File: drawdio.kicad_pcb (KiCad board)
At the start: 2 copper layers, 45.7 x 12.7 mm, 12 parts, among them P1 CONN_2, P2 CONN_01X01, Q1 BC558, Q2 BC547, U1 LM555N

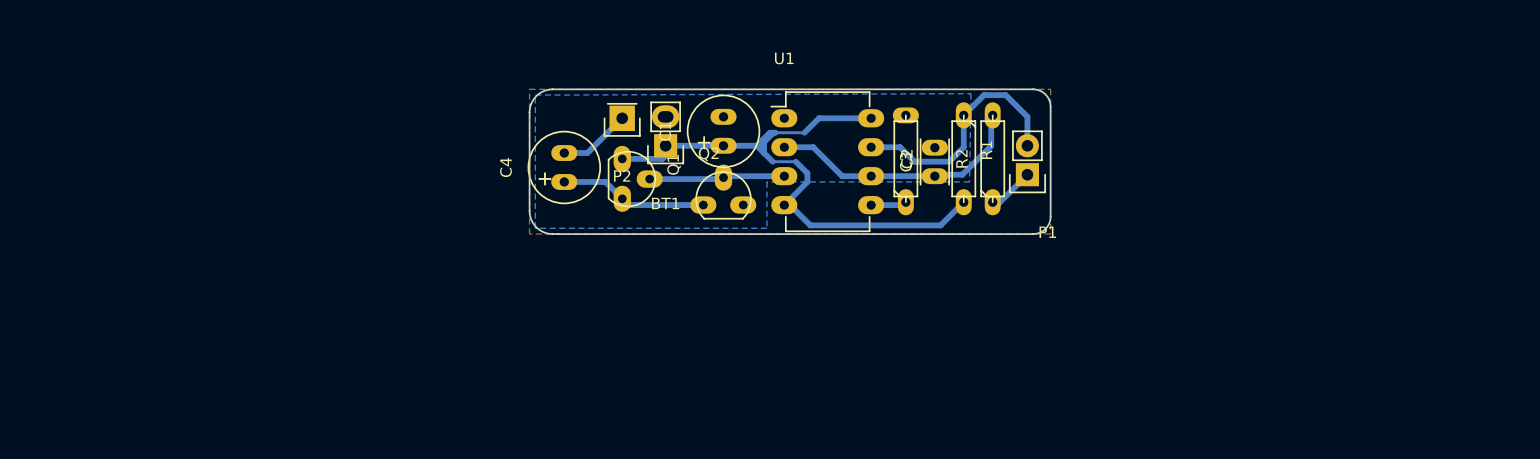
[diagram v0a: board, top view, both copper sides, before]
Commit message: Heavy work
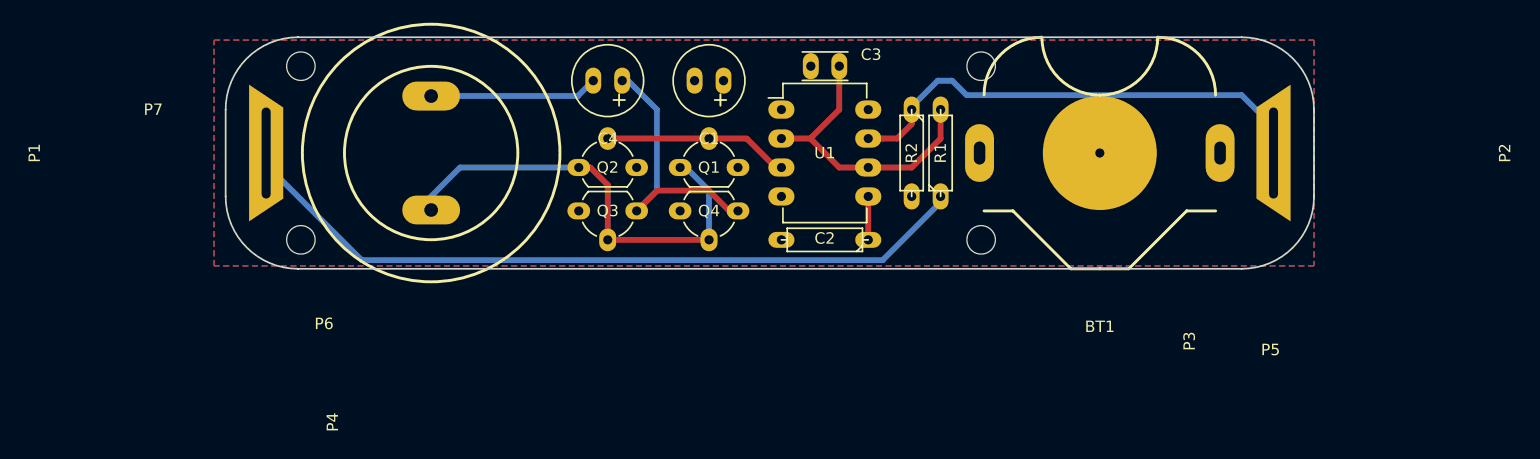
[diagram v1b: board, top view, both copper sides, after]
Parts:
- added P3: CONN_01X01, Mounting_Holes:MountingHole_2-5mm, F.Cu at (120.4, 94.0)
- added P4: CONN_01X02, drawdio:RS_mini_speaker_724-3100, F.Cu at (72.1, 86.4)
- added P5: CONN_01X01, Mounting_Holes:MountingHole_2-5mm, F.Cu at (120.4, 78.7)
- added P6: CONN_01X01, Mounting_Holes:MountingHole_2-5mm, F.Cu at (60.7, 94.0)
- added P7: CONN_01X01, Mounting_Holes:MountingHole_2-5mm, F.Cu at (60.7, 78.7)
- added Q3: BC558, Housings_TO-92:TO-92_Molded_Wide_Oval, F.Cu at (90.2, 91.4)
- added Q4: BC547, Housings_TO-92:TO-92_Molded_Wide_Oval, F.Cu at (99.1, 91.4)
- BT1: footprint Pin_Headers:Pin_Header_Straight_1x02 -> drawdio:CR2025_Keystone_3002_button_cell_holder_SMT
- P1: value CONN_2 -> CONN_01X01; footprint Pin_Headers:Pin_Header_Straight_1x02 -> drawdio:Drawdio_conn
- P2: footprint Pin_Headers:Pin_Header_Straight_1x01 -> drawdio:Drawdio_conn
- Q1, Q2: footprint drawdio:TO-92_JorFru_compact -> Housings_TO-92:TO-92_Molded_Wide_Oval
- moved P1 66.8 mm to (57.7, 86.4), turned to 270 degrees
- moved P2 57.2 mm to (146.1, 86.4), turned to 90 degrees
- moved BT1 38.1 mm to (130.8, 86.4), turned to 0 degrees
- moved C3 12.8 mm to (108.0, 78.7), turned to 180 degrees
- moved Q2 11.8 mm to (85.1, 87.6)
- moved C4 10.2 mm to (88.9, 80.0), turned to 180 degrees
- moved C2 10.1 mm to (106.7, 94.0), turned to 180 degrees
- moved C1 5.71 mm to (97.8, 80.0), turned to 180 degrees
- moved R1 4.60 mm to (116.8, 86.4)
- moved R2 4.60 mm to (114.3, 86.4)
- moved Q1 4.58 mm to (94.0, 87.6), turned to 0 degrees
- moved U1 0.80 mm to (102.9, 82.5)
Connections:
- P2 pad 1: Net-(C4-Pad2) -> Net-(P2-Pad1)
- Q1 pad 1: VCC -> Net-(P4-Pad2)
- Q1 pad 3: Net-(C4-Pad1) -> VCC
- Q2 pad 1: Net-(C4-Pad1) -> Net-(P4-Pad2)
- R2 pad 1: Net-(P1-Pad2) -> Net-(P2-Pad1)
- U1 pad 7: Net-(P1-Pad2) -> Net-(P2-Pad1)
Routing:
- net Net-(P1-Pad1): track 4.23 -> 66.7 mm
- net VCC: track 54.7 -> 0.00 mm
- net Net-(P2-Pad1): track 0.00 -> 50.9 mm
- net Net-(P4-Pad2): track 0.00 -> 40.2 mm
- net Net-(P1-Pad2): track 21.9 -> 0.00 mm
- net Net-(C4-Pad1): track 13.0 -> 24.1 mm
- net Net-(C4-Pad2): track 6.34 -> 15.8 mm
- net Net-(Q1-Pad2): track 13.3 -> 16.8 mm
- net Net-(C3-Pad1): track 23.6 -> 26.0 mm
- added copper zone on B.Cu, net VCC
- removed copper zone on B.Cu, net GND
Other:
- board size 45.7 x 12.7 mm -> 95.5 x 20.3 mm
